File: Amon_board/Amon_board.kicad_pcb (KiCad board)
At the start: 4 copper layers, 70 x 120 mm, 128 parts, among them J1 USB2.0_C_Rev, J10 GTFP08131Y2HR, J11 Conn_01x03_Male, J12 Conn_01x06_Male, J13 Conn_01x04_Male, J14 Conn_01x04_Male, J15 Conn_01x06_Male, J2 Conn_2x5 pin, J3 Switch_port, J4 XT60-F, J5 XT60-F, J6 Conn_02x04_Odd_Even, J7 Red leds, J8 White leds, J9 Conn_02x04_Odd_Even, M1 Servo_X+, M2 Servo_X-, M3 Servo_Y+, M4 Servo_Y-, Q1 BC817, Q2 BC817, SW1 SW_DPDT, SW2 SW_SPST, U1 USBLC6-2P6, U2 STM32F405RGT6-LQFP64, U3 W25Q128JVS, U4 MP2303ADN, U5 MP2303ADN, U6 MPU-6050, U7 BME280, U8 HMC5883L, Y1 25MHz

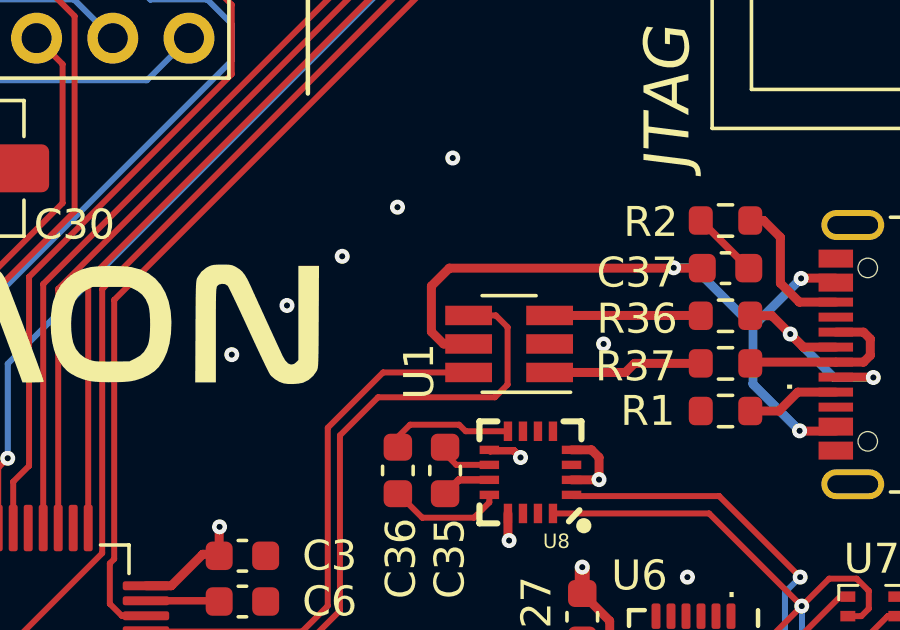
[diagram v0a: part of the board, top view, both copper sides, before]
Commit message: added pictires
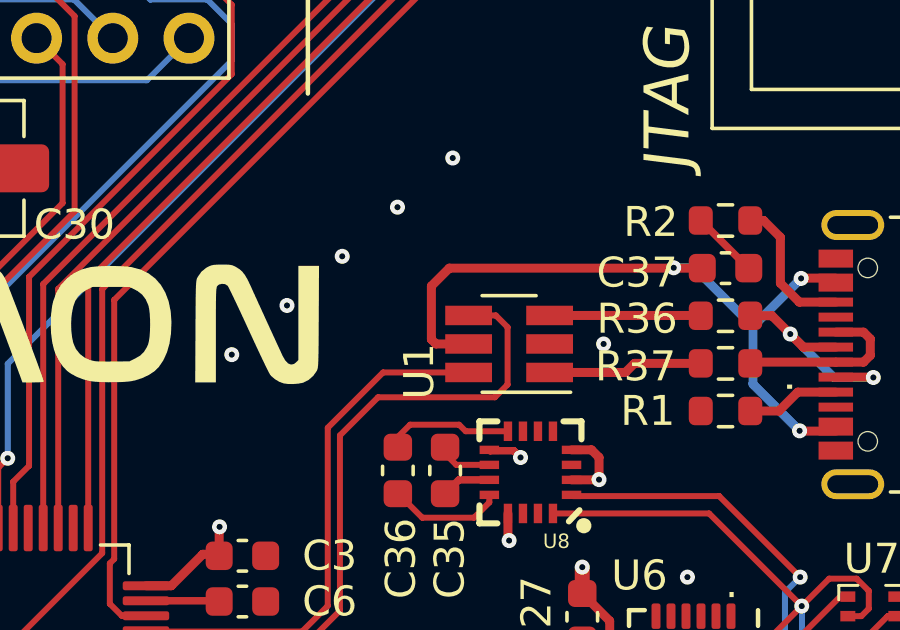
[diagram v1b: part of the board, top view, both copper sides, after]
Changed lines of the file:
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@@
   (segment (start 161.5652 107.412) (end 160.02 105.8668) (width 1) (layer "F.Cu") (net 14))
   (segment (start 167.4368 107.412) (end 161.5652 107.412) (width 1) (layer "F.Cu") (net 14))
+  (segment (start 205.232 78.1304) (end 205.3844 78.2828) (width 0.3) (layer "F.Cu") (net 15))
+  (segment (start 205.232 76.3524) (end 205.232 78.1304) (width 0.3) (layer "F.Cu") (net 15))
   (segment (start 217.5058 81.1784) (end 217.5158 81.1884) (width 0.3) (layer "F.Cu") (net 15))
   (segment (start 213.3219 75.7555) (end 213.3092 75.7428) (width 0.3) (layer "F.Cu") (net 15))
-  (segment (start 205.232 76.3524) (end 205.232 77.8764) (width 0.3) (layer "F.Cu") (net 15))
-  (segment (start 205.232 77.8764) (end 205.6384 78.2828) (width 0.3) (layer "F.Cu") (net 15))
   (segment (start 217.5566 76.0984) (end 217.5666 76.0884) (width 0.3) (layer "F.Cu") (net 15))
-  (segment (start 213.3092 75.7428) (end 213.2965 75.7555) (width 0.3) (layer "F.Cu") (net 15))
+  (segment (start 205.3844 78.2828) (end 206.4728 78.2828) (width 0.3) (layer "F.Cu") (net 15))
   (segment (start 214.2614 75.7555) (end 213.3219 75.7555) (width 0.3) (layer "F.Cu") (net 15))
   (segment (start 217.5158 81.1884) (end 218.7126 81.1884) (width 0.3) (layer "F.Cu") (net 15))
+  (segment (start 213.3092 75.7428) (end 213.2965 75.7555) (width 0.3) (layer "F.Cu") (net 15))
   (segment (start 217.5666 76.0884) (end 218.7126 76.0884) (width 0.3) (layer "F.Cu") (net 15))
-  (segment (start 205.6384 78.2828) (end 206.4728 78.2828) (width 0.3) (layer "F.Cu") (net 15))
   (segment (start 213.2965 75.7555) (end 205.8289 75.7555) (width 0.3) (layer "F.Cu") (net 15))
   (segment (start 205.8289 75.7555) (end 205.232 76.3524) (width 0.3) (layer "F.Cu") (net 15))
